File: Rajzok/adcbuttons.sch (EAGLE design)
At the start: 17 parts, among them Q1 TP0602N2, Q2 TP0602N2, Q3 SUP75N06-08, Q4 SUP75N06-08

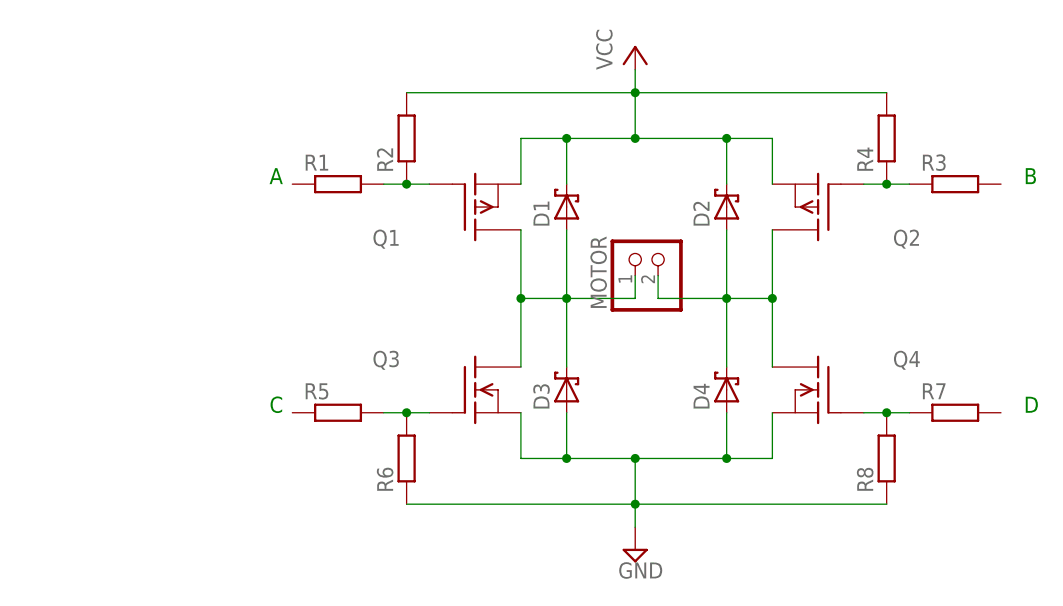
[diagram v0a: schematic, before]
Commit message: Rajzok 2017
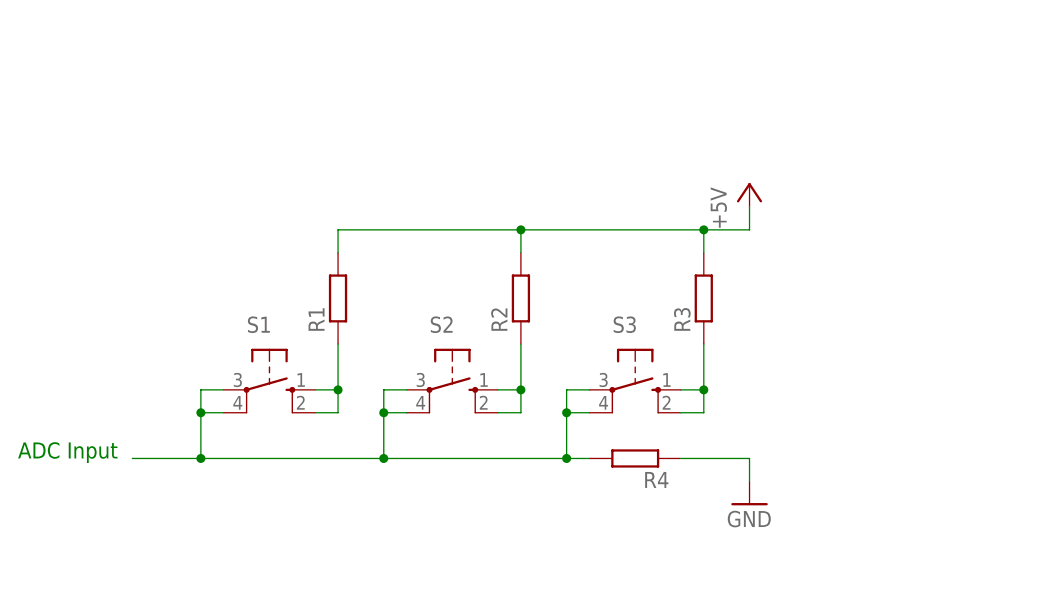
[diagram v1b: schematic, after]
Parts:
- removed D1, D2, D3, D4: 1N6267A, diode:1N6267A
- removed MOTOR: (no value), pinhead:PINHD-1X2
- removed Q1, Q2: TP0602N2, transistor-fet:TP0602N2
- removed Q3, Q4: SUP75N06-08, transistor-fet:SUP75N06-08
- removed R5, R6, R7, R8: (no value), rcl:R-EU_0204/7
- added S1, S2, S3: (no value), switch-omron:10-XX
- R1, R2, R3, R4: device rcl:R-EU_0204/7 -> rcl:R-EU_0309/10
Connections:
- removed net N$2: D2.A, D4.C, MOTOR.2, Q2.D, Q4.D
- removed net N$3: Q2.G, R3.1, R4.1
- removed net N$9: D1.A, D3.C, MOTOR.1, Q1.D, Q3.D
- removed net VCC: D1.C, D2.C, Q1.S, Q2.S, R2.2, R4.2
- new net +5V: R1.2, R2.2, R3.2
- new net N$6: R3.1, S3.S, S3.S1
- net GND: now also R4.1; no longer D3.A, D4.A, Q3.S, Q4.S, R6.1, R8.1
- net N$1: now also R4.2, S1.P, S1.P1, S2.P, S2.P1, S3.P, S3.P1; no longer Q1.G, R1.2, R2.1
- net N$4: now also R1.1, S1.S, S1.S1; no longer Q3.G, R5.2, R6.2
- net N$5: now also R2.1, S2.S, S2.S1; no longer Q4.G, R7.1, R8.2
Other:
- note added: "ADC Input"
- note removed: "A"
- note removed: "B"
- note removed: "C"
- note removed: "D"
- moved on the sheet: R1, R2, R3, R4
